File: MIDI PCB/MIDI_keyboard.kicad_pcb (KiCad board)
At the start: 2 copper layers, 101 x 76 mm, 11 parts, among them J1 Capactitive Touch Buttons, SW2 SW_Push, U1 XIAO-ESP32-S3

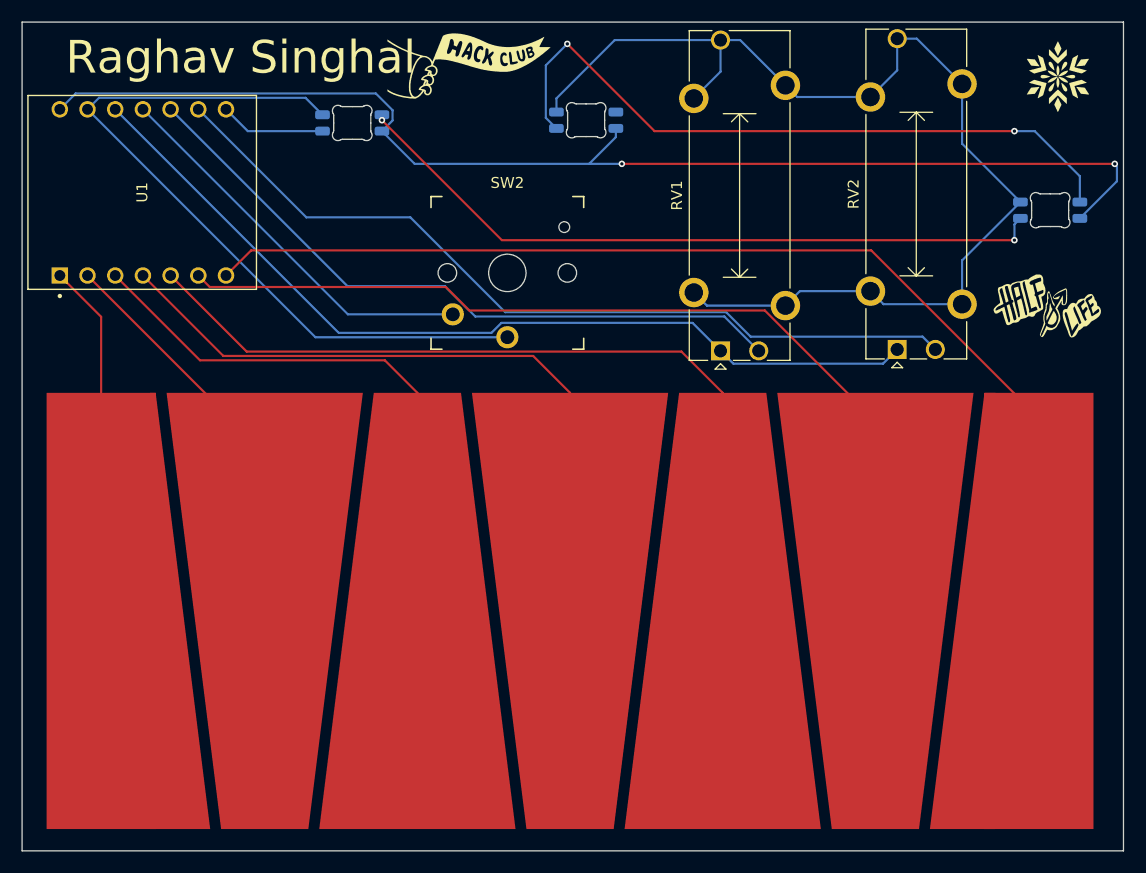
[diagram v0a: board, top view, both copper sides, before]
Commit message: fixed pcb
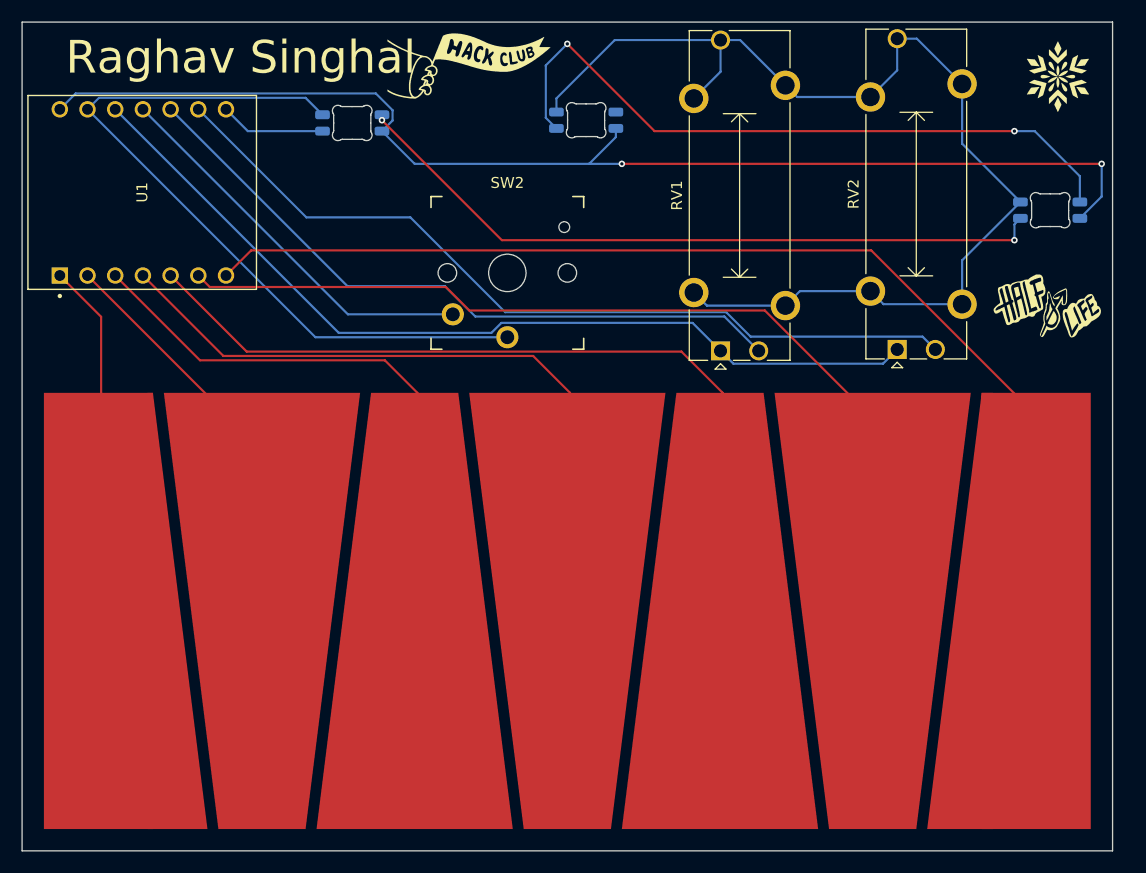
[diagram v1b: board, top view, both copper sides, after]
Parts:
- moved J1 0.25 mm to (127.0, 103.0)
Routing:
- net +5V: track 113.4 -> 111.4 mm
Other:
- board size 101 x 76 mm -> 100 x 76 mm
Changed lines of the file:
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@@
 	(footprint "raghav:Capacitive Keys"
 		(layer "F.Cu")
-		(at 127.25 103)
+		(at 127 103)
 		(property "Reference" "J1"
 			(at 13.75 -6 0)
@@
 	(gr_rect
 		(start 128 69)
-		(end 229 145)
+		(end 228 145)
 		(radius 3)
 		(stroke
@@
 	)
 	(segment
-		(start 228.2 82)
+		(start 227 82)
 		(end 183 82)
 		(width 0.2)
@@
 	)
 	(via
-		(at 228.2 82)
+		(at 227 82)
 		(size 0.6)
 		(drill 0.3)
@@
 	)
 	(segment
-		(start 228.4 83.6)
-		(end 228.4 82)
+		(start 225 87)
+		(end 227 85)
 		(width 0.2)
 		(layer "B.Cu")
@@
 	)
 	(segment
-		(start 225 87)
-		(end 228.4 83.6)
+		(start 227 85)
+		(end 227 82)
 		(width 0.2)
 		(layer "B.Cu")
@@
 		(width 0.2)
 		(layer "B.Cu")
-		(net "+5V")
-	)
-	(segment
-		(start 228.4 82)
-		(end 228.2 82)
-		(width 0.2)
-		(layer "B.Cu")
